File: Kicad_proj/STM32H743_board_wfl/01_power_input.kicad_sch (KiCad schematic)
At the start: 5 parts

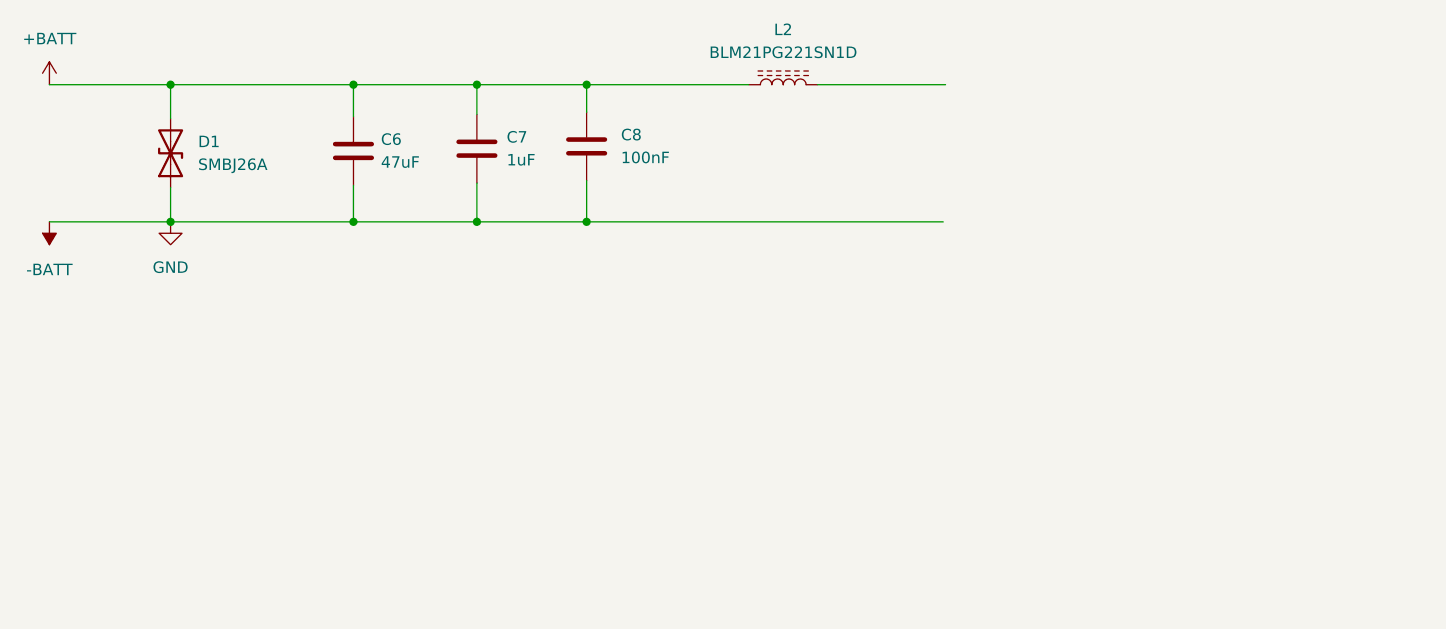
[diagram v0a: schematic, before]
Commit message: v0.4 poprawki inputa zasilania
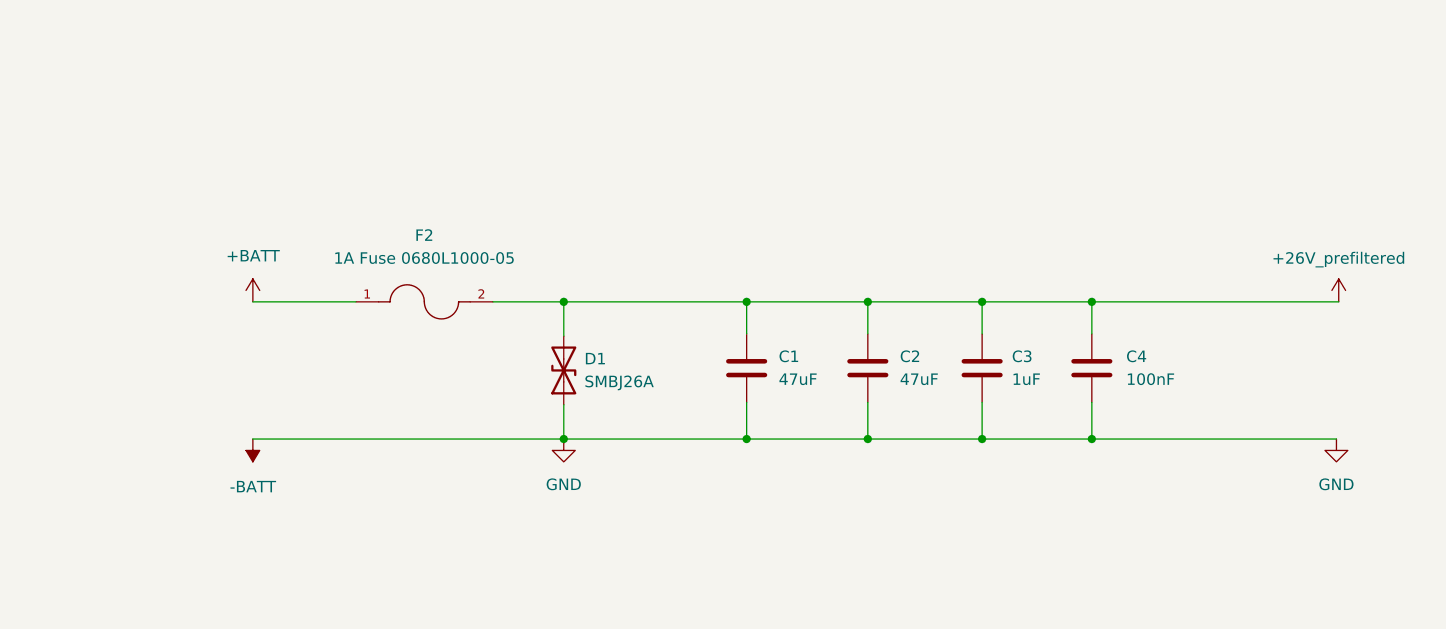
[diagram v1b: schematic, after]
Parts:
- removed C6: 47uF, symbol Device:C
- removed C7: 1uF, symbol Device:C
- removed C8: 100nF, symbol Device:C
- removed L2: BLM21PG221SN1D, symbol Device:L_Ferrite
- added C1, C2: 47uF, Capacitor_SMD:C_1206_3216Metric, symbol Device:C
- added C3: 1uF, Capacitor_SMD:C_0603_1608Metric, symbol Device:C
- added C4: 100nF, Capacitor_SMD:C_01005_0402Metric, symbol Device:C
- added F2: 1A Fuse 0680L1000-05, STM32H743_board_library_footprints:FUSC6125X279N, symbol STM32H743_board_library_symbols:0680L1000-05
- D1: footprint (none) -> Diode_SMD:D_SMB
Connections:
- net +BATT: now also F2.1; no longer D1.2 (A2)
- net -BATT: now also C1.2, C2.2, C3.2, C4.2
- new net +26V_prefiltered: C1.1, C2.1, C3.1, C4.1, D1.2 (A2), F2.2

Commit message: v0.5 schematics + lib update
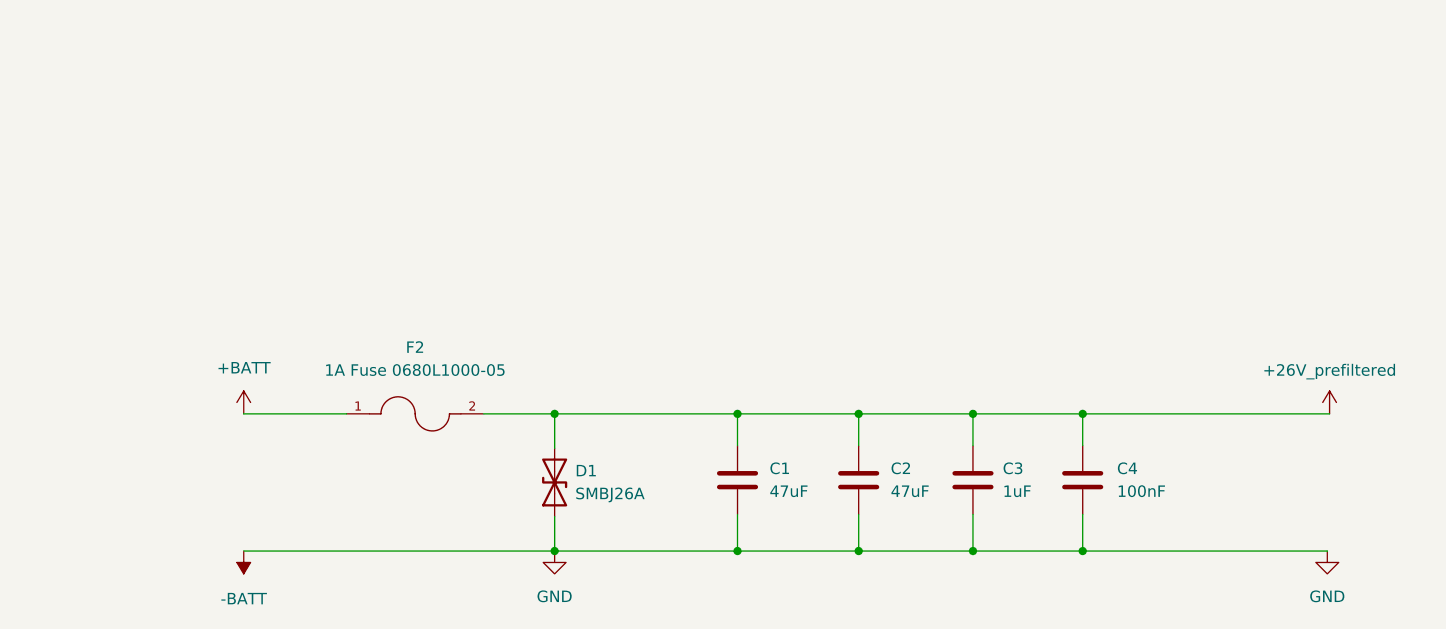
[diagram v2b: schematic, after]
